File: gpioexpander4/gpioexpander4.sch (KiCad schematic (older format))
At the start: 21 parts, among them J1 PWR, J2 I2C, J3 Port 1, J4 Port 2, J5 Port 3, J6 Port 4, J7 Port 5, J8 ~INT, SW1 Action, U1 MCP23017-E/SP

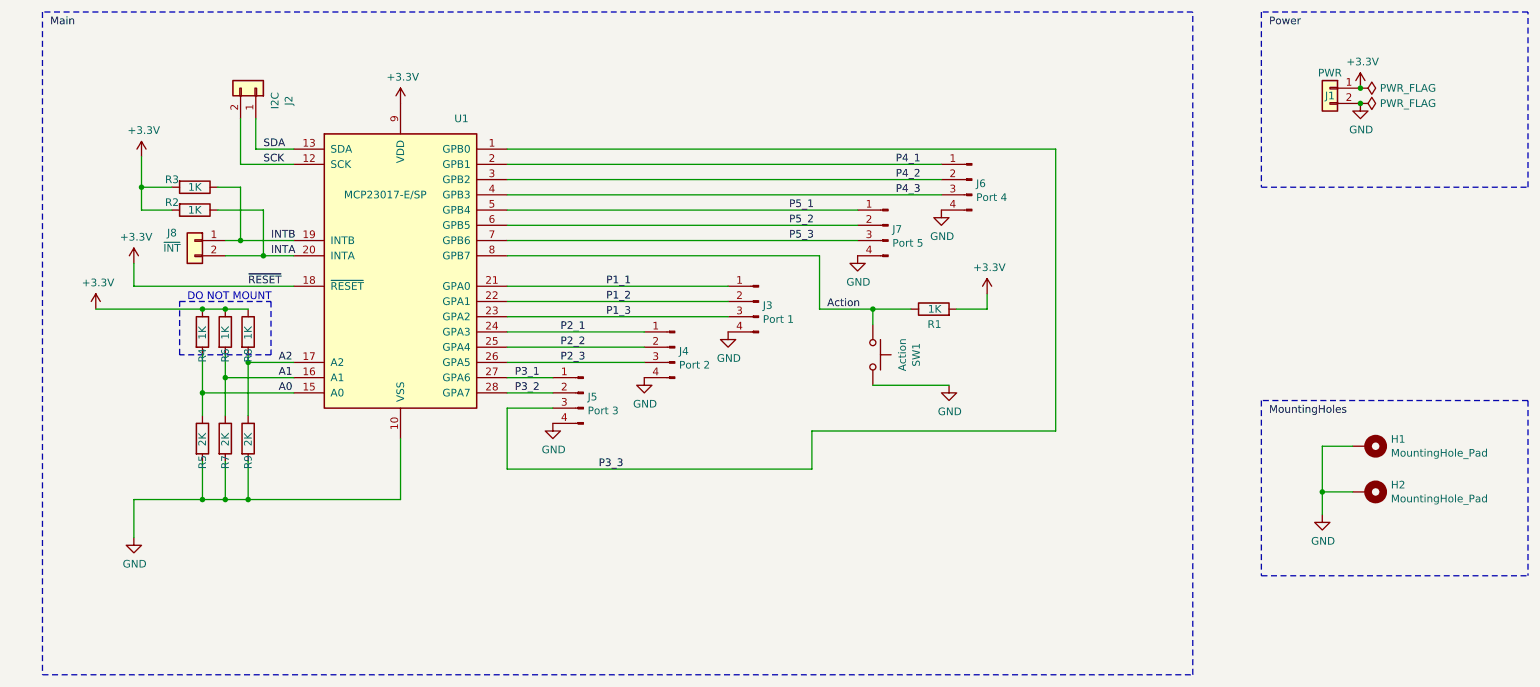
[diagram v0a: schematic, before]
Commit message: Production run 1
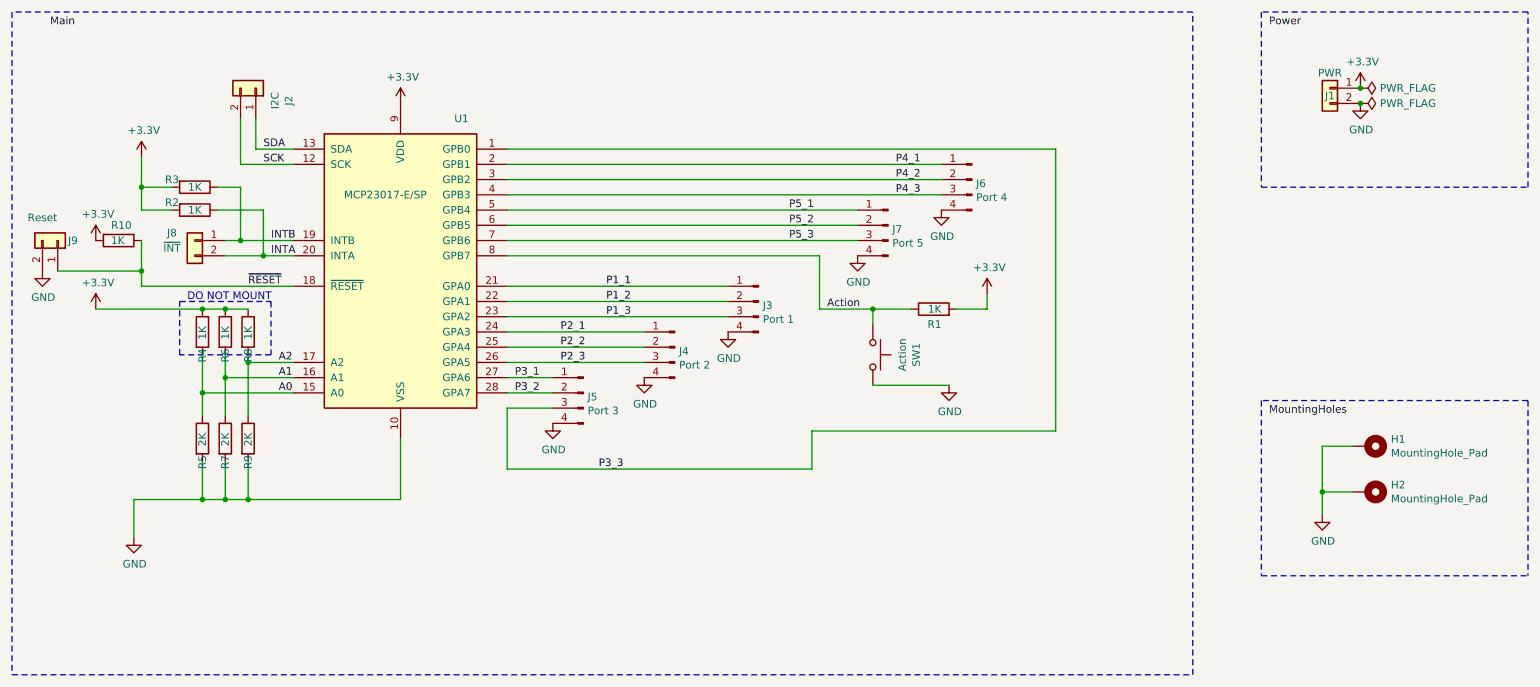
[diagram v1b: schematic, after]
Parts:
- added J9: Reset, Connector_PinHeader_2.54mm:PinHeader_1x02_P2.54mm_Vertical, symbol Connector_Generic:Conn_01x02
- added R10: 1K, Resistor_SMD:R_0805_2012Metric_Pad1.15x1.40mm_HandSolder, symbol Device:R
- H1, H2: footprint MountingHole:MountingHole_4.3mm_M4_Pad -> MountingHole:MountingHole_3.2mm_M3_Pad
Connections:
- net +3V3: now also R10.2; no longer U1.18 (~RESET~)
- net GND: now also J9.2 (Pin_2)
- new net ~RESET: J9.1 (Pin_1), R10.1, U1.18 (~RESET~)
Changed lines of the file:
@@
 F 0 "H1" V 9604 4050 50  0000 L CNN
 F 1 "MountingHole_Pad" V 9695 4050 50  0000 L CNN
-F 2 "MountingHole:MountingHole_4.3mm_M4_Pad" H 9650 3900 50  0001 C CNN
+F 2 "MountingHole:MountingHole_3.2mm_M3_Pad" H 9650 3900 50  0001 C CNN
 F 3 "~" H 9650 3900 50  0001 C CNN
 	1    9650 3900
@@
 F 0 "H2" V 9604 4350 50  0000 L CNN
 F 1 "MountingHole_Pad" V 9695 4350 50  0000 L CNN
-F 2 "MountingHole:MountingHole_4.3mm_M4_Pad" H 9650 4200 50  0001 C CNN
+F 2 "MountingHole:MountingHole_3.2mm_M3_Pad" H 9650 4200 50  0001 C CNN
 F 3 "~" H 9650 4200 50  0001 C CNN
 	1    9650 4200
@@
 	10700 3600 10700 4750
 Wire Notes Line
-	950  1050 950  5400
-Wire Notes Line
-	950  5400 8500 5400
+	750  1050 750  5400
+Wire Notes Line
+	750  5400 8500 5400
 Wire Notes Line
 	8500 5400 8500 1050
 Wire Notes Line
-	8500 1050 950  1050
+	8500 1050 750  1050
 Wire Notes Line
 	8950 2200 10700 2200
@@
 	2400 2650 2150 2650
 Wire Wire Line
-	2600 2850 1550 2850
+	2600 2850 1600 2850
 Wire Wire Line
 	1600 2350 1800 2350
@@
 Wire Wire Line
 	6950 3000 7150 3000
-$Comp
-L power:+3.3V #PWR0113
-U 1 1 5F647715
-P 1550 2700
-F 0 "#PWR0113" H 1550 2550 50  0001 C CNN
-F 1 "+3.3V" H 1565 2873 50  0000 C CNN
-F 2 "" H 1550 2700 50  0001 C CNN
-F 3 "" H 1550 2700 50  0001 C CNN
-	1    1550 2700
-	1    0    0    -1
-$EndComp
-Wire Wire Line
-	1550 2850 1550 2700
 Wire Wire Line
 	1600 2000 1600 2200
@@
 Text Label 2400 2050 0    50   ~ 0
 SCK
+Wire Wire Line
+	1600 2850 1600 2750
+$Comp
+L power:+3.3V #PWR0113
+U 1 1 5F647715
+P 1300 2550
+F 0 "#PWR0113" H 1300 2400 50  0001 C CNN
+F 1 "+3.3V" H 1315 2723 50  0000 C CNN
+F 2 "" H 1300 2550 50  0001 C CNN
+F 3 "" H 1300 2550 50  0001 C CNN
+	1    1300 2550
+	1    0    0    -1
+$EndComp
+$Comp
+L Device:R R10
+U 1 1 5F6402C1
+P 1450 2550
+F 0 "R10" V 1350 2500 50  0000 L CNN
+F 1 "1K" V 1450 2500 50  0000 L CNN
+F 2 "Resistor_SMD:R_0805_2012Metric_Pad1.15x1.40mm_HandSolder" V 1380 2550 50  0001 C CNN
+F 3 "~" H 1450 2550 50  0001 C CNN
+F 4 "DNF" H 1450 2550 50  0001 C CNN "DNF"
+	1    1450 2550
+	0    1    1    0
+$EndComp
+$Comp
+L Connector_Generic:Conn_01x02 J9
+U 1 1 5F644F9E
+P 1050 2550
+F 0 "J9" V 1050 2650 50  0000 C CNN
+F 1 "Reset" V 1200 2450 50  0000 C CNN
+F 2 "Connector_PinHeader_2.54mm:PinHeader_1x02_P2.54mm_Vertical" H 1050 2550 50  0001 C CNN
+F 3 "~" H 1050 2550 50  0001 C CNN
+	1    1050 2550
+	0    1    -1   0
+$EndComp
+Wire Wire Line
+	1050 2750 1600 2750
+Connection ~ 1600 2750
+Wire Wire Line
+	1600 2750 1600 2550
+$Comp
+L power:GND #PWR?
+U 1 1 5F64D986
+P 950 2750
+F 0 "#PWR?" H 950 2500 50  0001 C CNN
+F 1 "GND" H 955 2577 50  0000 C CNN
+F 2 "" H 950 2750 50  0001 C CNN
+F 3 "" H 950 2750 50  0001 C CNN
+	1    950  2750
+	1    0    0    -1
+$EndComp
 $EndSCHEMATC
